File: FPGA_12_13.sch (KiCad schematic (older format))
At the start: 5 parts, among them U1 XC7K160T-FFG676, U51 TXB0104D

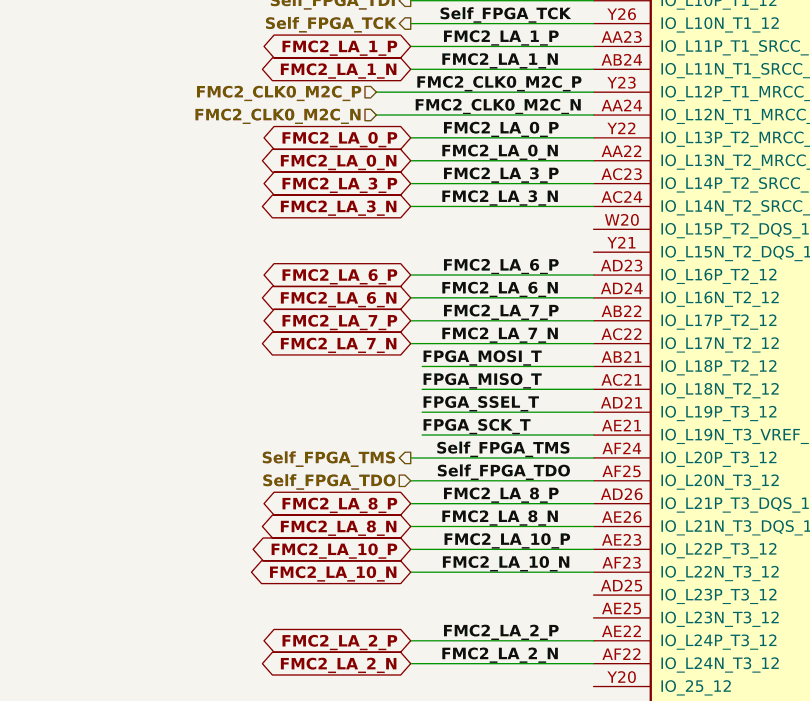
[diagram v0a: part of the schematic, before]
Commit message: routing done
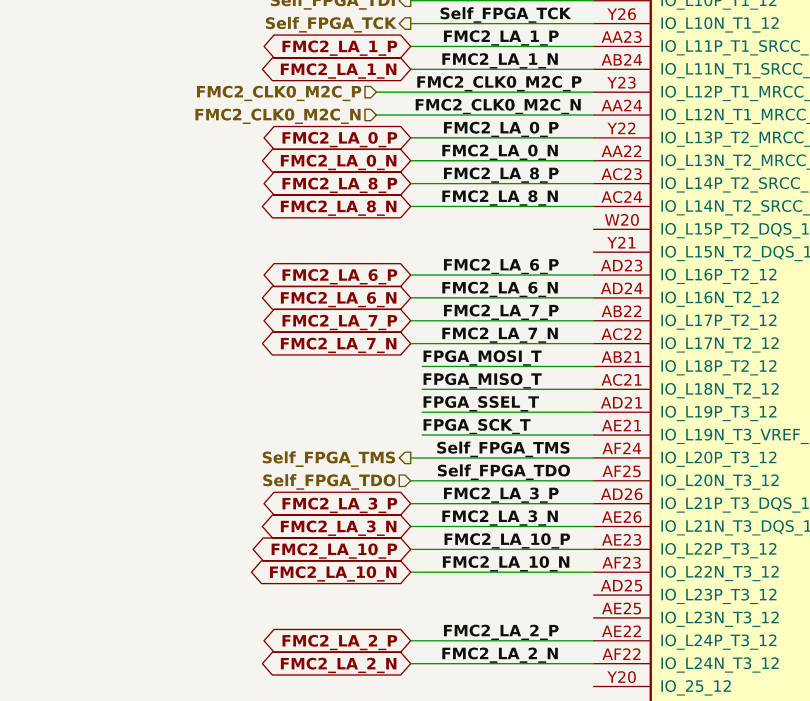
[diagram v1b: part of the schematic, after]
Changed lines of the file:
@@
 Text Label 6450 5650 2    50   ~ 10
 FMC2_LA_0_N
-Text Label 6450 5750 2    50   ~ 10
+Text Label 6450 7150 2    50   ~ 10
 FMC2_LA_3_P
 Text Label 6450 4750 2    50   ~ 10
@@
 Text Label 6500 3150 2    50   ~ 10
 FMC2_LA_15_P
-Text Label 6450 5850 2    50   ~ 10
+Text Label 6450 7250 2    50   ~ 10
 FMC2_LA_3_N
 Text Label 6450 4850 2    50   ~ 10
@@
 	5800 7850 6600 7850
 Wire Wire Line
-	5800 5750 6600 5750
-Wire Wire Line
-	5800 5850 6600 5850
+	5800 7150 6600 7150
+Wire Wire Line
+	5800 7250 6600 7250
 Wire Wire Line
 	5800 4750 6600 4750
@@
 Text GLabel 5800 7850 0    50   BiDi ~ 10
 FMC2_LA_2_N
-Text GLabel 5800 5750 0    50   BiDi ~ 10
+Text GLabel 5800 7150 0    50   BiDi ~ 10
 FMC2_LA_3_P
-Text GLabel 5800 5850 0    50   BiDi ~ 10
+Text GLabel 5800 7250 0    50   BiDi ~ 10
 FMC2_LA_3_N
 Text GLabel 5800 4750 0    50   BiDi ~ 10
@@
 Text GLabel 5800 4050 0    50   BiDi ~ 10
 FMC2_LA_16_N
-Text Label 6450 7250 2    50   ~ 10
-FMC2_LA_8_N
-Wire Wire Line
-	5800 7150 6600 7150
-Wire Wire Line
-	5800 7250 6600 7250
-Text GLabel 5800 7150 0    50   BiDi ~ 10
-FMC2_LA_8_P
-Text GLabel 5800 7250 0    50   BiDi ~ 10
-FMC2_LA_8_N
 Wire Wire Line
 	5800 3150 6600 3150
@@
 	1    0    0    -1
 $EndComp
-Text Label 6450 7150 2    50   ~ 10
-FMC2_LA_8_P
 $Comp
 L Resistors_SMD:R0402_0R_JUMPER R?
@@
 	3400 4150 3250 4150
 Connection ~ 3400 4150
+Text Label 6450 5850 2    50   ~ 10
+FMC2_LA_8_N
+Wire Wire Line
+	5800 5750 6600 5750
+Wire Wire Line
+	5800 5850 6600 5850
+Text GLabel 5800 5750 0    50   BiDi ~ 10
+FMC2_LA_8_P
+Text GLabel 5800 5850 0    50   BiDi ~ 10
+FMC2_LA_8_N
+Text Label 6450 5750 2    50   ~ 10
+FMC2_LA_8_P
 $EndSCHEMATC
